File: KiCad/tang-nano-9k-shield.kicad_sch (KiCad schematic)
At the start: 68 parts, among them J1 Barrel_Jack, J2 AudioJack3, J3 USB_A_Stacked, J5 DE15_Socket_HighDensity_Mount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, Q1 SS8050, U1 Tang Nano 9K, U3 TPS563201DDCR, U4 AMS1117-3.3, U5 PT8211, U6 TPA6132A2RTE, U7 USBLC6-2SC6, U8 USBLC6-2SC6

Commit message: Add files via upload
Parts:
- removed J3: USB_A_Stacked, symbol Connector:USB_A_Stacked
- removed U8: USBLC6-2SC6, Package_TO_SOT_SMD:SOT-23-6, symbol Power_Protection:USBLC6-2SC6
- added C1, C21: 20pF, symbol Device:C_Small
- added C25, C26, C27, C28, C29, C30: 100nF, symbol Device:C_Small
- added D3, D4: SS14, Diode_SMD:D_SMA, symbol Diode:SS14
- added J3: USB_C_Receptacle_USB2.0_16P, symbol Connector:USB_C_Receptacle_USB2.0_16P
- added J6: DE9_Socket_MountingHoles, symbol Connector:DE9_Socket_MountingHoles
- added JP1: SolderJumper_2_Open, symbol Jumper:SolderJumper_2_Open
- added JP2: RST, symbol Jumper:SolderJumper_2_Open
- added R30: 10K, symbol Device:R_Small
- added R31, R32: 5K1, symbol Device:R_Small
- added U10: MAX3232, symbol Interface_UART:MAX3232
- added U8: RP2040, Package_DFN_QFN:QFN-56-1EP_7x7mm_P0.4mm_EP3.2x3.2mm, symbol MCU_RaspberryPi:RP2040
- added U9: W25Q32JVZP, Package_SON:WSON-8-1EP_6x5mm_P1.27mm_EP3.4x4.3mm, symbol Memory_Flash:W25Q32JVZP
- added Y1: X322512MSB4SI, symbol Device:Crystal_GND23_Small
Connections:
- net 3V3: now also C23.2, C25.2, R30.1, U10.16 (VCC), U8.1 (IOVDD), U8.10 (IOVDD), U8.22 (IOVDD), U8.33 (IOVDD), U8.42 (IOVDD), U8.43 (ADC_AVDD), U8.44 (VREG_VIN), U8.48 (USB_VDD), U8.49 (IOVDD), U9.8 (VCC)
- net 5V: now also D3.1 (K), D4.1 (K); no longer C23.1, C6.1, C7.1, L1.2, R7.1
- net D1+: now also U8.47 (USB_DP)
- net D1-: now also U8.46 (USB_DM)
- net GND: now also C23.1, C1.1, C21.1, C25.1, C26.1, C29.2, C30.2, J3.A1 (GND), J3.A12 (GND), J3.B1 (GND), J3.B12 (GND), J3.SH (SHIELD), J6.5, J6.SH (PAD), JP1.1 (A), JP2.1 (A), R31.2, R32.2, U10.15 (GND), U8.57 (GND), U9.4 (GND), U9.9 (EP), Y1.2 (G), Y1.3 (G); no longer C23.2
- net RAW_D1+: now also J3.A6 (D+), J3.B6 (D+)
- net RAW_D1-: now also J3.A7 (D-), J3.B7 (D-)
- net SCK: now reaches U1.28 (IOB11B)
- net SCK: now also U8.29 (GPIO18)
- net MOSI: now reaches U1.29 (IOB13A)
- net MOSI: now also U8.27 (GPIO16)
- net MISO: now reaches U1.30 (IOB13B)
- net MISO: now also U8.30 (GPIO19)
- net CS1: now reaches U1.33 (IOB23A)
- net CS1: now also U8.28 (GPIO17)
- net INT1: now reaches U1.34 (IOB23B)
- net INT1: now also U8.31 (GPIO20)
- net RS_RX: now reaches U1.36 (IOB29B)
- net RS_RX: now also U10.12 (R1OUT)
- net RS_TX: now reaches U1.37 (IOB31A)
- net RS_TX: now also U10.11 (T1IN)
- new net: C28.1, U10.4 (C2+)
- new net: C28.2, U10.5 (C2-)
- new net: C26.2, U8.23 (DVDD), U8.45 (VREG_VOUT), U8.50 (DVDD)
- new net: JP2.2 (B), R30.2, U8.26 (RUN)
- new net: U8.51 (QSPI_SD3), U9.7 (~{HOLD}/~{RESET}/IO_{3})
- new net: U8.52 (QSPI_SCLK), U9.6 (CLK)
- new net: U8.53 (QSPI_SD0), U9.5 (DI/IO_{0})
- new net: U8.54 (QSPI_SD2), U9.3 (~{WP}/IO_{2})
- new net: U8.55 (QSPI_SD1), U9.2 (DO/IO_{1})
- new net: J3.A5 (CC1), R31.1
- new net: C29.1, U10.2 (VS+)
- new net: C30.1, U10.6 (VS-)
- new net: J3.B5 (CC2), R32.1
- new net: C27.1, U10.1 (C1+)
- new net: C27.2, U10.3 (C1-)
- new net 5V_BUCK: C6.1, C7.1, D4.2 (A), L1.2, R7.1
- new net 5V_USB: D3.2 (A), J3.A4 (VBUS), J3.A9 (VBUS), J3.B4 (VBUS), J3.B9 (VBUS)
- new net BOOTSEL: JP1.2 (B), U8.56 (~{QSPI_SS}), U9.1 (~{CS})
- new net RXD: J6.2, U10.14 (T1OUT)
- new net TXD: J6.3, U10.13 (R1IN)
- new net XIN: C1.2, U8.20 (XIN), Y1.1
- new net XOUT: C21.2, U8.21 (XOUT), Y1.4
- no-connect marks 10 -> 50
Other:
- note added: "RP 2040"
- note added: "RS-232"
- note added: "USB-C"
- moved on the sheet: BZ1, C10, C11, C12, C13, C14, C15, C16, C17, C18, C19, C2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

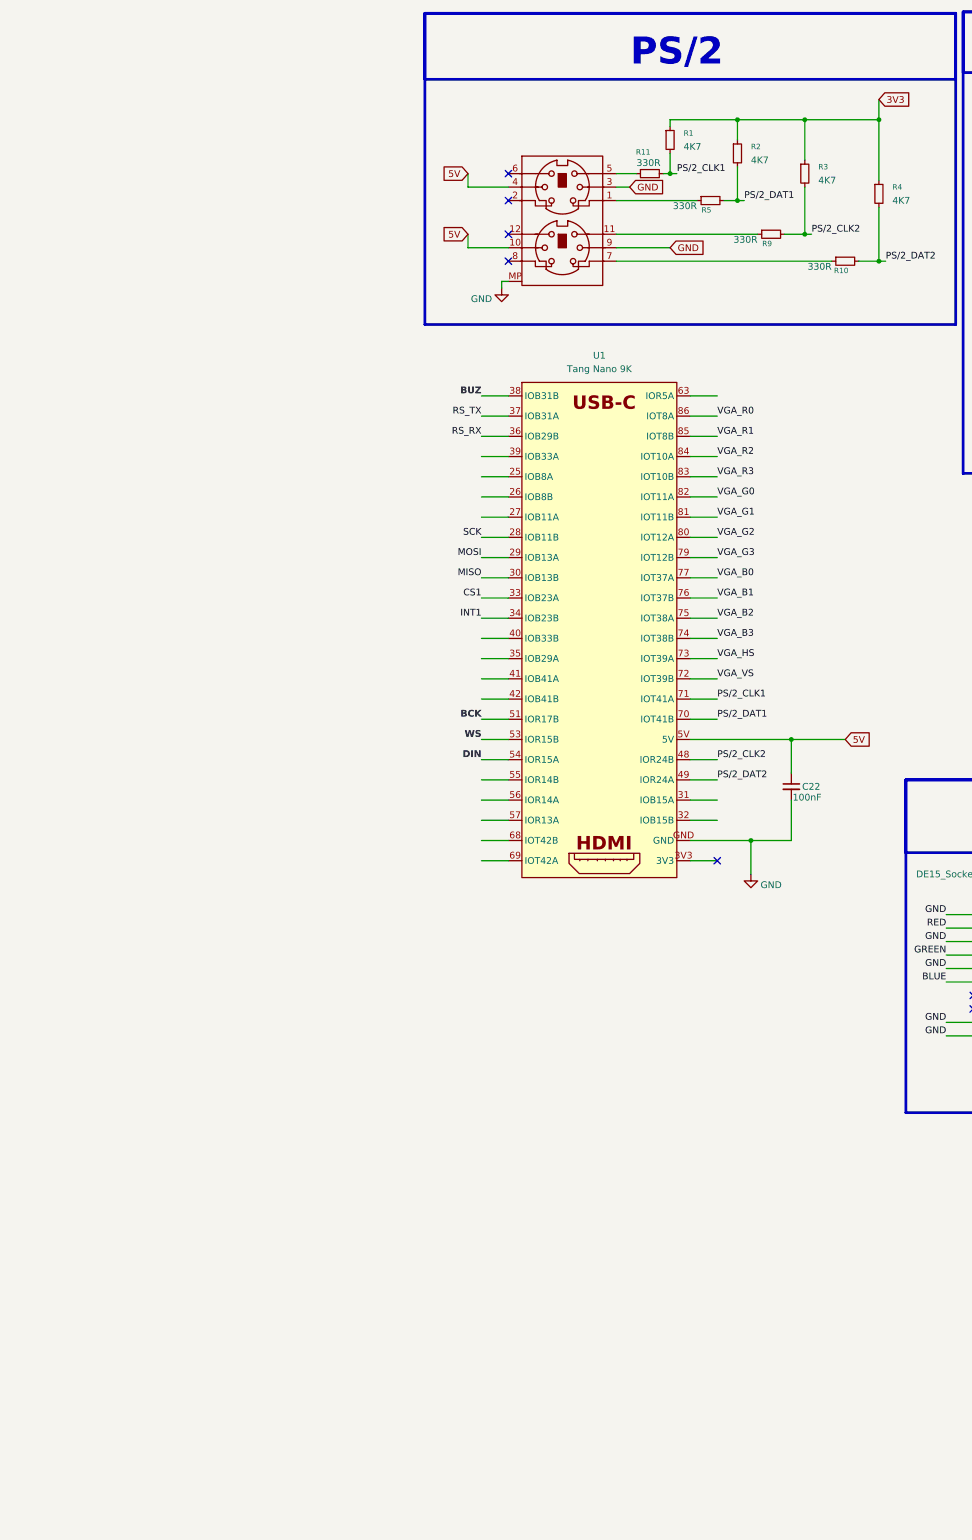
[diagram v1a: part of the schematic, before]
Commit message: Add files via upload
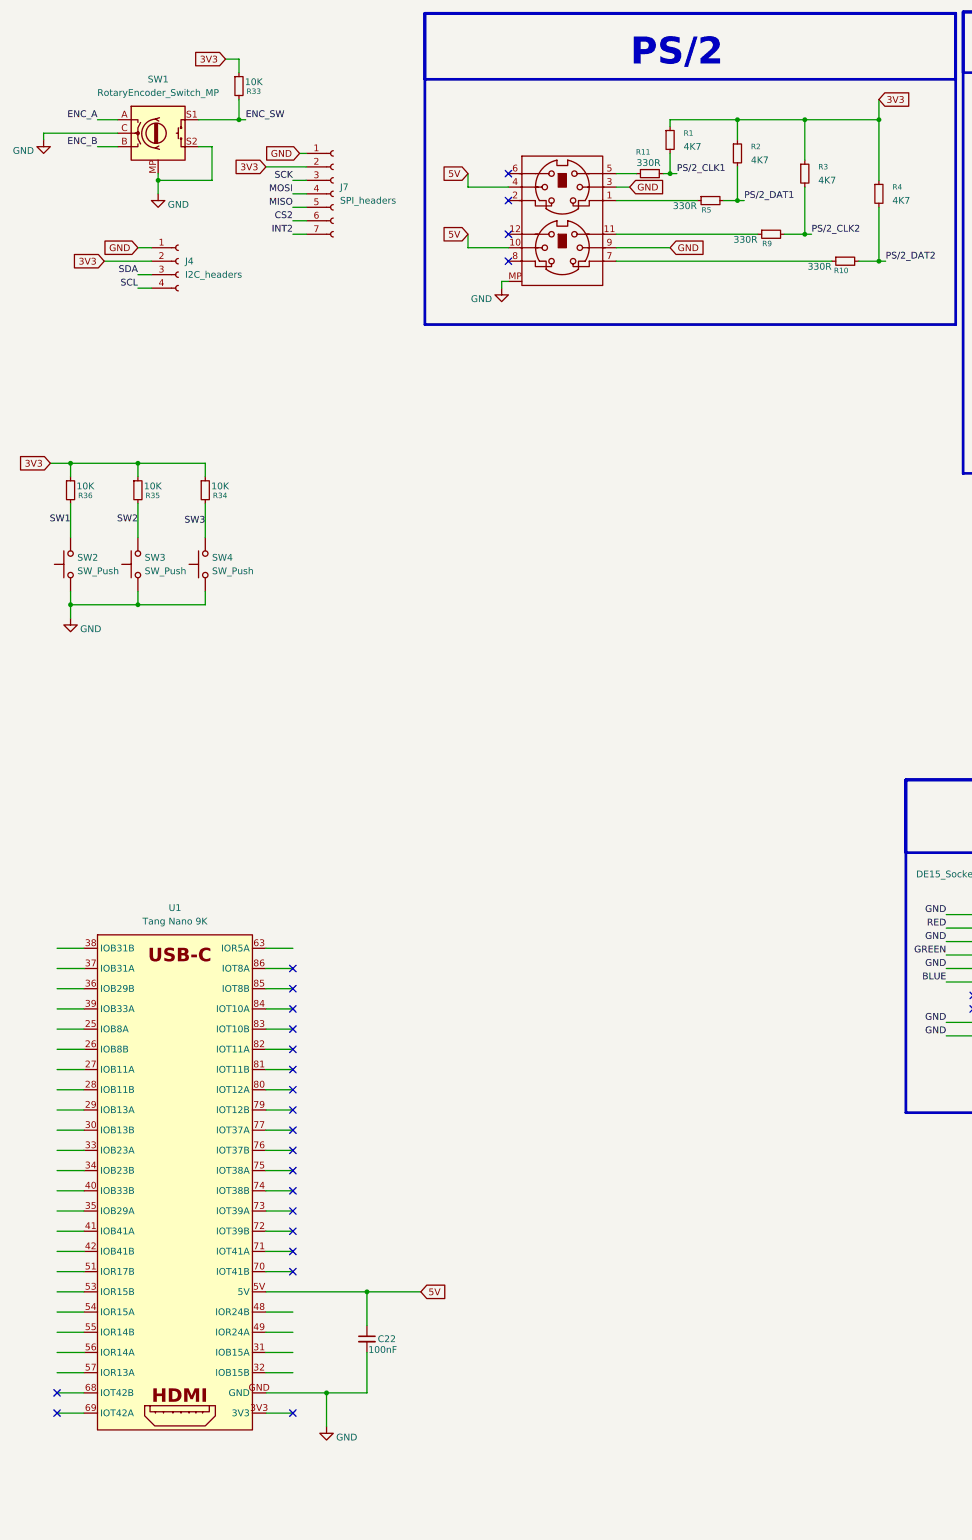
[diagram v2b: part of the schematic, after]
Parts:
- added J4: I2C_headers, symbol Connector:Conn_01x04_Socket
- added J7: SPI_headers, symbol Connector:Conn_01x07_Socket
- added R33, R34, R35, R36: 10K, symbol Device:R_Small
- added SW1: RotaryEncoder_Switch_MP, symbol Device:RotaryEncoder_Switch_MP
- added SW2, SW3, SW4: SW_Push, symbol Switch:SW_Push
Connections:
- net 3V3: now also J4.2 (Pin_2), J7.2 (Pin_2), R33.1, R34.1, R35.1, R36.1
- net BCK: no longer U1.51 (IOR17B)
- net BUZ: no longer U1.38 (IOB31B)
- net CS1: no longer U1.33 (IOB23A)
- net DIN: no longer U1.54 (IOR15A)
- net GND: now also J4.1 (Pin_1), J7.1 (Pin_1), SW1.C, SW1.MP, SW1.S2, SW2.1, SW3.1, SW4.1
- net INT1: no longer U1.34 (IOB23B)
- net MISO: now also J7.5 (Pin_5); no longer U1.30 (IOB13B)
- net MOSI: now also J7.4 (Pin_4); no longer U1.29 (IOB13A)
- net PS/2_CLK1: no longer U1.71 (IOT41A)
- net PS/2_CLK2: no longer U1.48 (IOR24B)
- net PS/2_DAT1: no longer U1.70 (IOT41B)
- net PS/2_DAT2: no longer U1.49 (IOR24A)
- net RS_RX: no longer U1.36 (IOB29B)
- net RS_TX: no longer U1.37 (IOB31A)
- net SCK: now also J7.3 (Pin_3); no longer U1.28 (IOB11B)
- net VGA_B0: no longer U1.77 (IOT37A)
- net VGA_B1: no longer U1.76 (IOT37B)
- net VGA_B2: no longer U1.75 (IOT38A)
- net VGA_B3: no longer U1.74 (IOT38B)
- net VGA_G0: no longer U1.82 (IOT11A)
- net VGA_G1: no longer U1.81 (IOT11B)
- net VGA_G2: no longer U1.80 (IOT12A)
- net VGA_G3: no longer U1.79 (IOT12B)
- net VGA_HS: no longer U1.73 (IOT39A)
- net VGA_R0: no longer U1.86 (IOT8A)
- net VGA_R1: no longer U1.85 (IOT8B)
- net VGA_R2: no longer U1.84 (IOT10A)
- net VGA_R3: no longer U1.83 (IOT10B)
- net VGA_VS: no longer U1.72 (IOT39B)
- net WS: no longer U1.53 (IOR15B)
- new net CS2: J7.6 (Pin_6)
- new net ENC_A: SW1.A
- new net ENC_B: SW1.B
- new net ENC_SW: R33.2, SW1.S1
- new net INT2: J7.7 (Pin_7)
- new net SCL: J4.4 (Pin_4)
- new net SDA: J4.3 (Pin_3)
- new net SW1: R36.2, SW2.2
- new net SW2: R35.2, SW3.2
- new net SW3: R34.2, SW4.2
- no-connect marks 50 -> 68
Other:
- moved on the sheet: C22, U1
